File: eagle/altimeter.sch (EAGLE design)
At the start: 34 parts, among them U1 328P

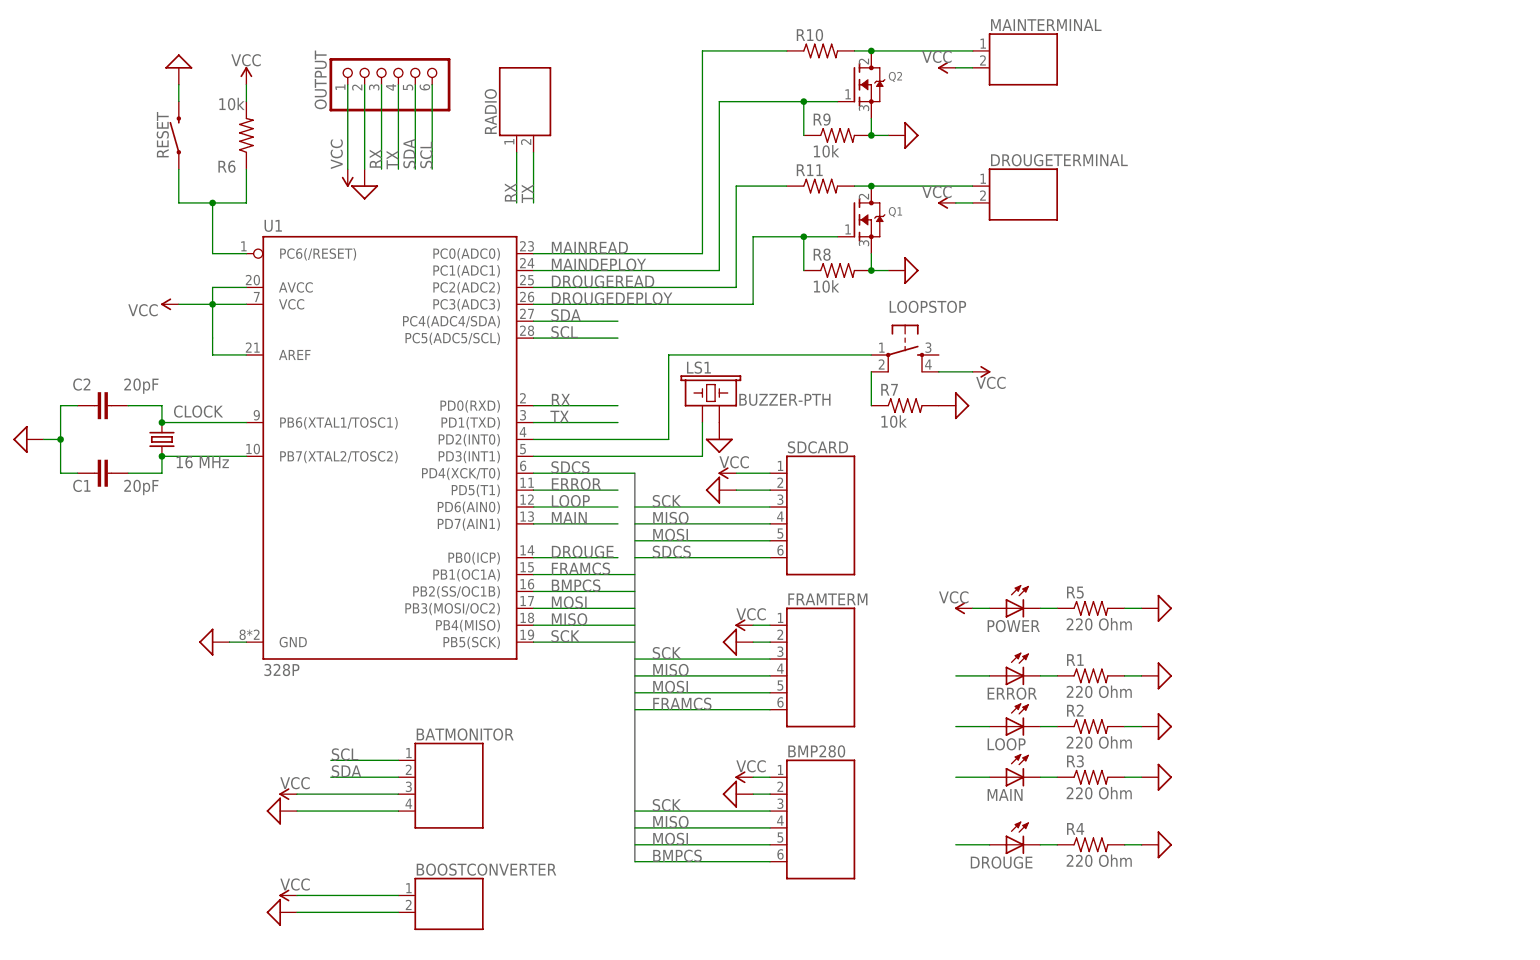
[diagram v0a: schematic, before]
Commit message: Created project structure and updated eagle files
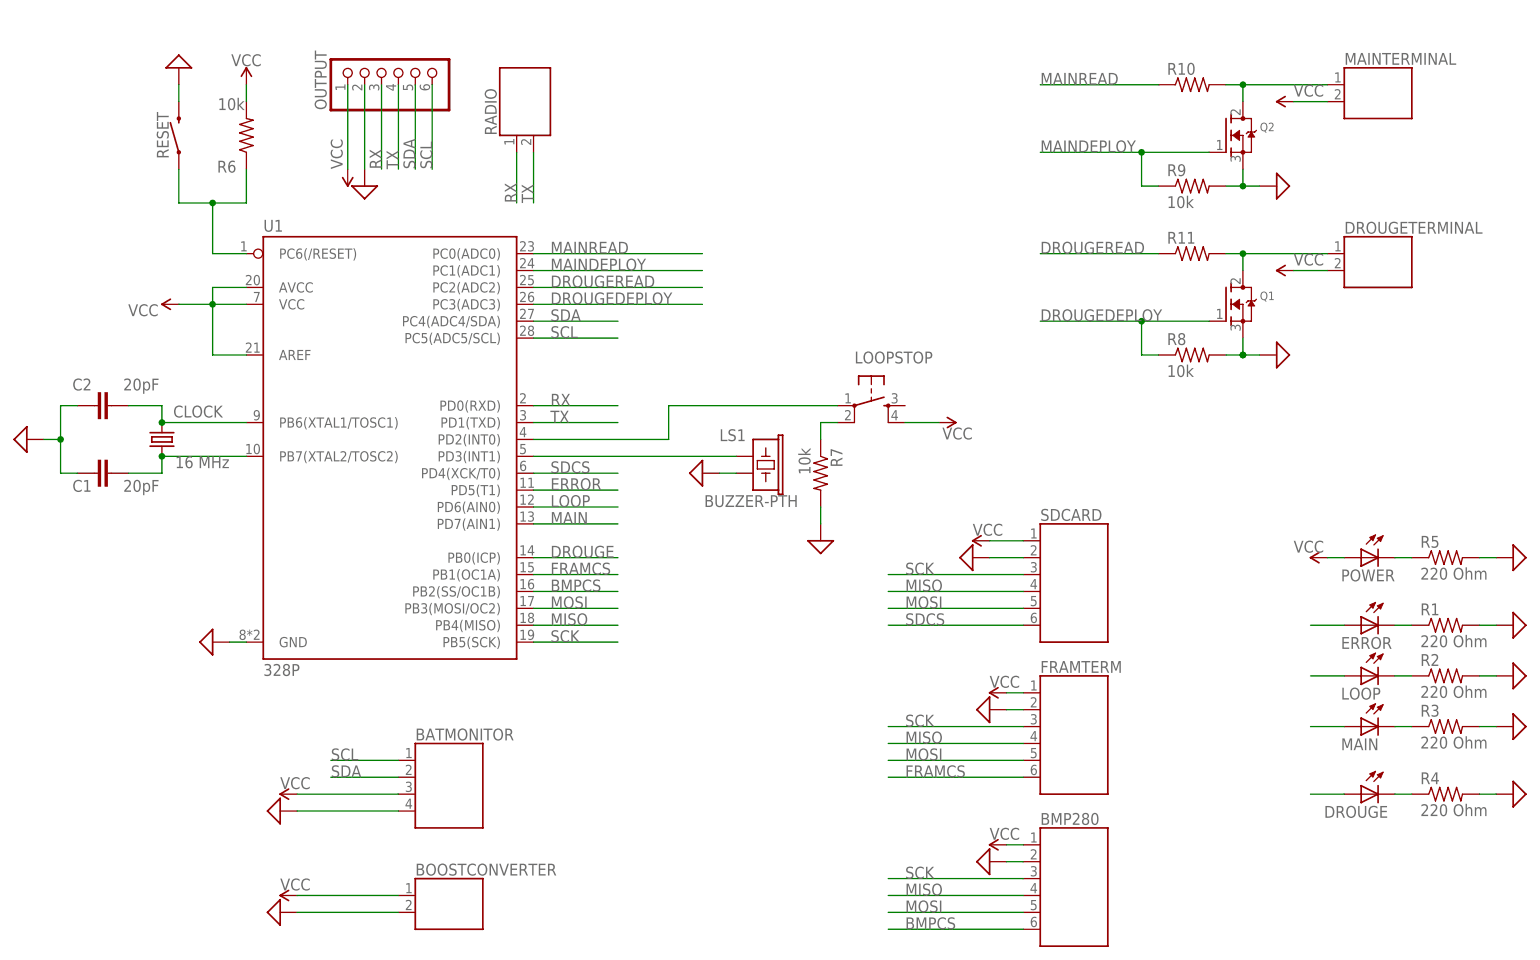
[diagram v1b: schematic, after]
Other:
- moved on the sheet: BMP280, DROUGE, DROUGETERMINAL, ERROR, FRAMTERM, LOOP, LOOPSTOP, LS1, MAIN, MAINTERMINAL, POWER, Q1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
